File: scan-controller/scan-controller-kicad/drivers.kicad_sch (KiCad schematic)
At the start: 40 parts, among them CN2 Motor, CN3 Fan, CN4 Lamp, Q1 IRF7470, Q8 SS8050, U3 78L05, U4 DRV8871DDA, U6 TL431, U7 XL4015, U8 LM358

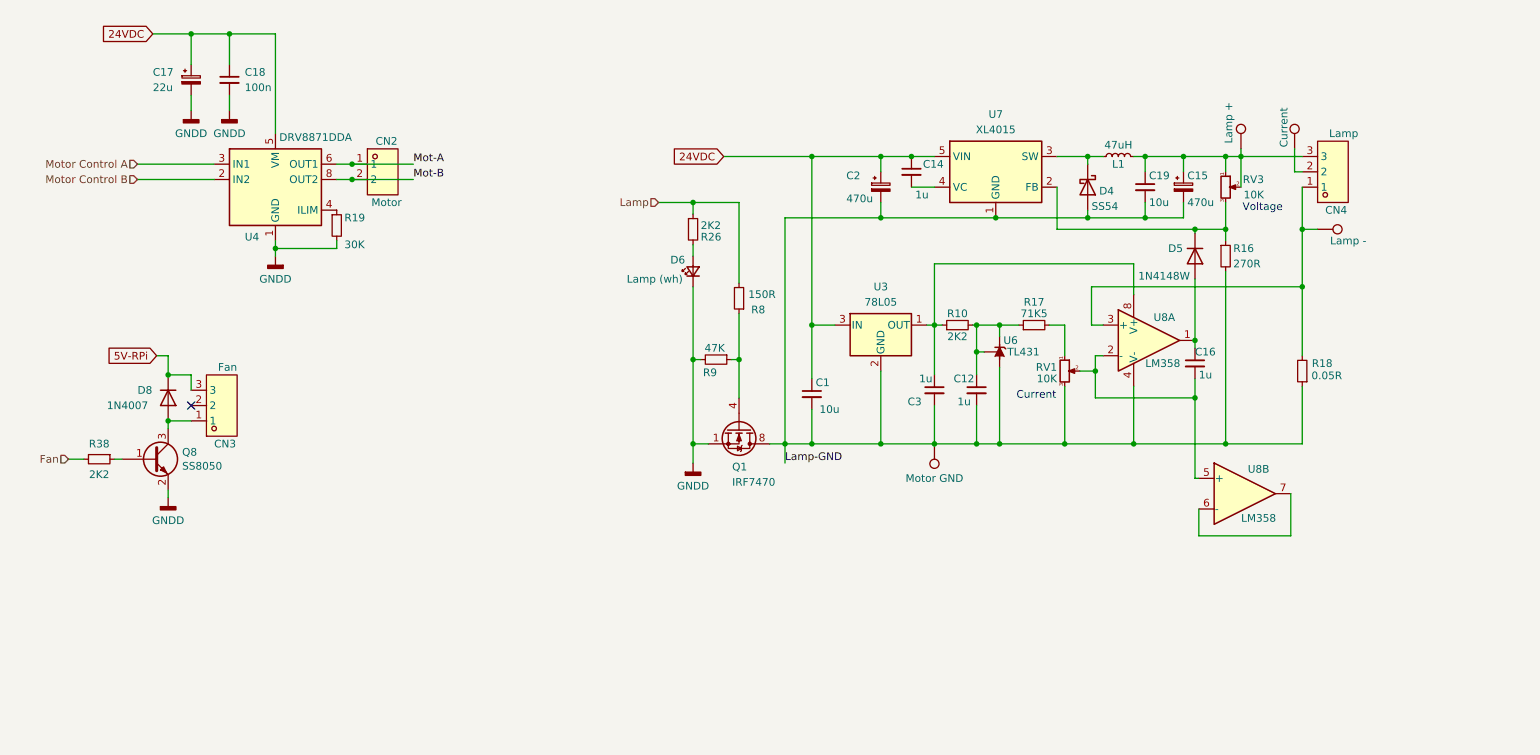
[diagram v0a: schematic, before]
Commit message: Adding a new Fan Driver (3-13V, 1A)
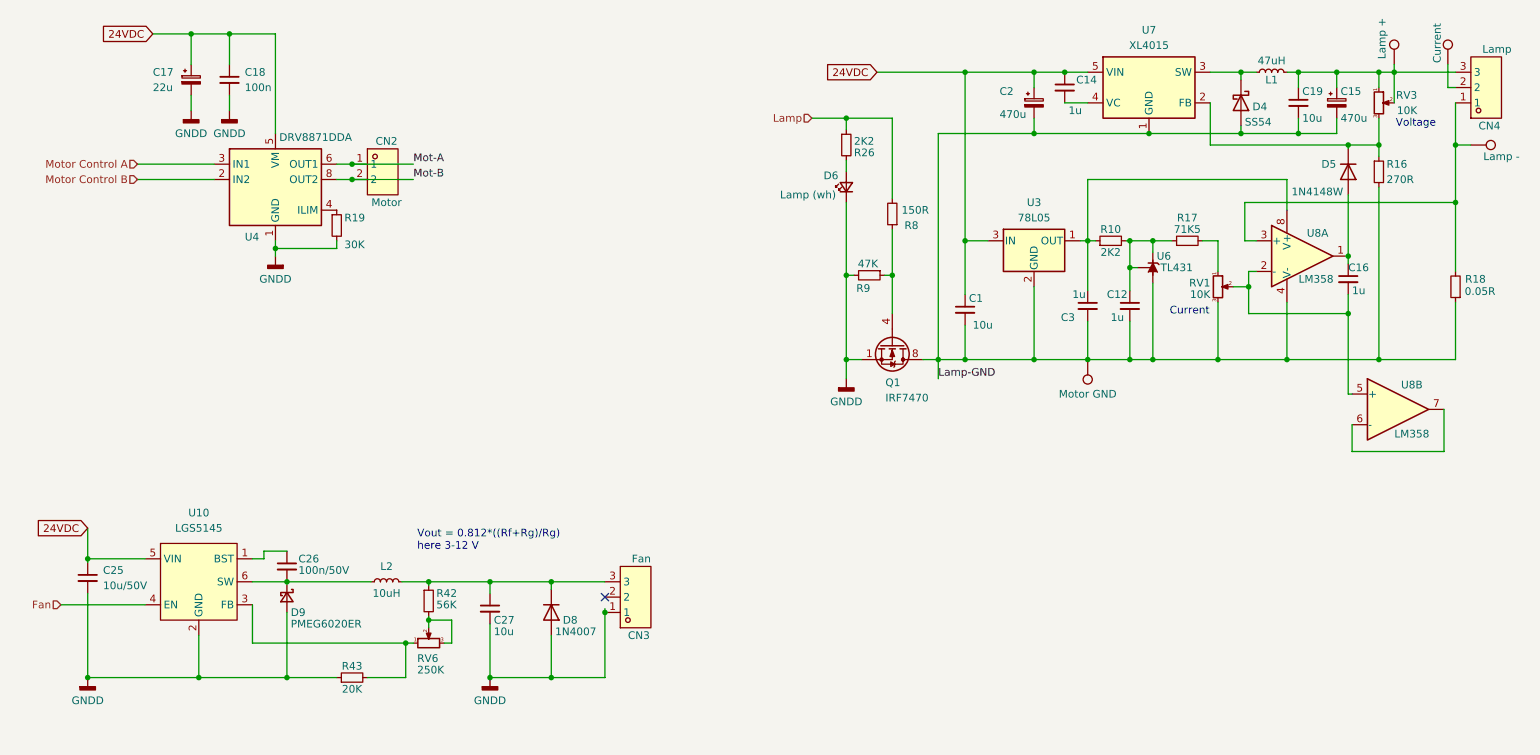
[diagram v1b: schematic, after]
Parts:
- removed Q8: SS8050, Package_TO_SOT_SMD:SOT-23, symbol Transistor_BJT:BC847
- removed R38: 2K2, Resistor_SMD:R_0805_2012Metric, symbol Device:R_Small
- added C25: 10u/50V, Capacitor_SMD:C_1210_3225Metric, symbol Device:C_Small
- added C26: 100n/50V, Capacitor_SMD:C_0805_2012Metric, symbol Device:C_Small
- added C27: 10u, Capacitor_SMD:C_0805_2012Metric, symbol Device:C_Small
- added D9: PMEG6020ER, Diode_SMD:D_SOD-123F, symbol Device:D_Schottky_Small
- added L2: 10uH, easyeda2kicad:IND-SMD_L4.4-W4.2, symbol Device:L_Small
- added R42: 56K, Resistor_SMD:R_0805_2012Metric, symbol Device:R_Small
- added R43: 20K, Resistor_SMD:R_0805_2012Metric, symbol Device:R_Small
- added RV6: 250K, easyeda2kicad:RES-ADJ-TH_3P-L10.0-W10.0-P2.50-L, symbol Device:R_Potentiometer_Small
- added U10: LGS5145, easyeda2kicad:SOT-23-6_L2.9-W1.7-P0.95-LS2.8-BL, symbol easyeda2kicad:LGS5145
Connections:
- net 24VDC: now also C25.1, U10.5 (VIN)
- net Fan: now also U10.4 (EN)
- net GNDD: now also CN3.1, D8.2 (A), C25.2, C27.2, D9.2 (A), R43.1, U10.2 (GND)
- net 5V-RPi: no longer names the net of CN3.3, D8.1 (K)
- net 5V-RPi: now also C27.1, L2.2, R42.1
- new net: C26.2, D9.1 (K), L2.1, U10.6 (SW)
- new net: R43.2, RV6.1, U10.3 (FB)
- new net: R42.2, RV6.2, RV6.3
- new net: C26.1, U10.1 (BST)
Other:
- note added: "Vout = 0.812*((Rf+Rg)/Rg) here 3-12 V"
- moved on the sheet: C1, C12, C14, C15, C16, C19, C2, C3, CN3, CN4, D4, D5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

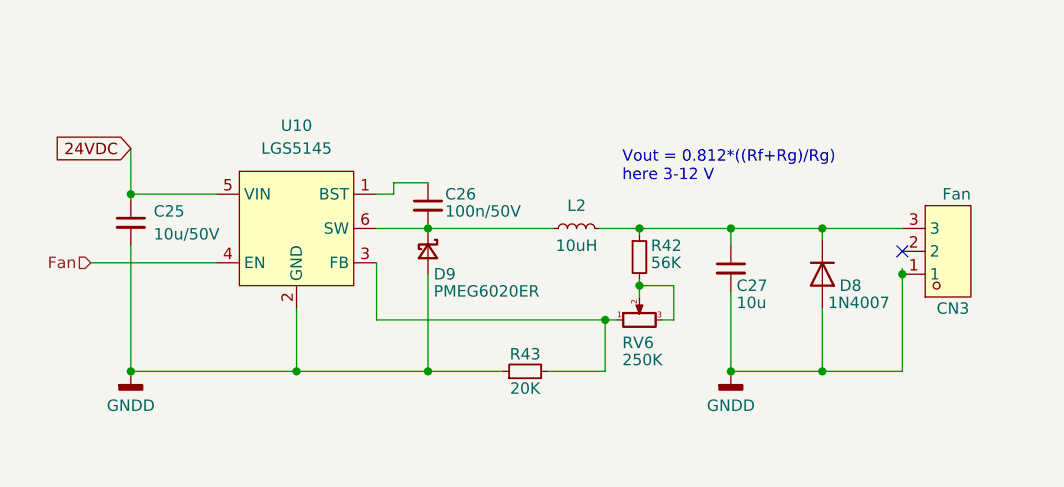
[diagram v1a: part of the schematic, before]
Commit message: Routing WIP
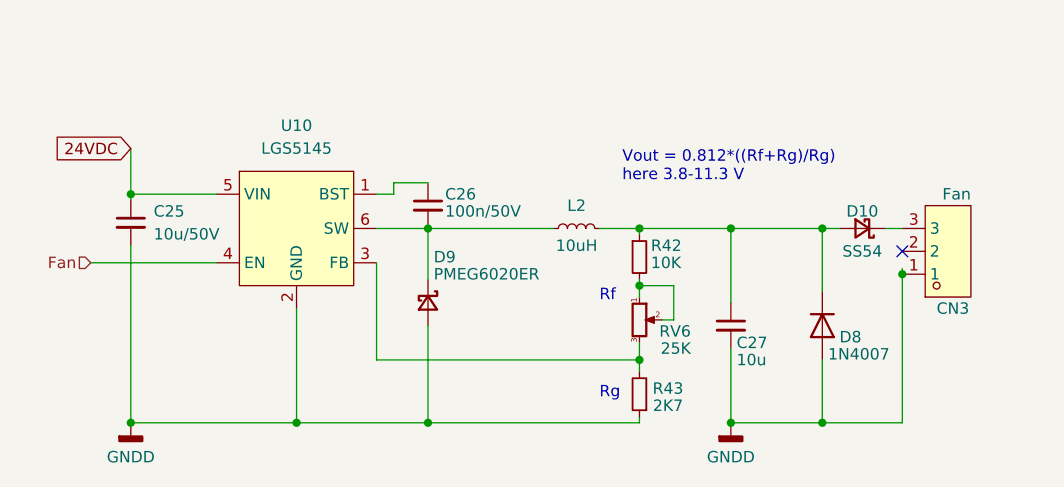
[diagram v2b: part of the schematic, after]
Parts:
- added D10: SS54, Diode_SMD:D_SMA, symbol Device:D_Schottky_Small
- R42: value 56K -> 10K; Inventory P -> B; LCSC C17756 -> C17414
- R43: value 20K -> 2K7; LCSC C4328 -> C17530
- RV6: value 250K -> 25K; LCSC C83691 -> C118932
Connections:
- net at C27.1, D8.1 (K), L2.2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: now also D10.2 (A); no longer CN3.3
- net at R43.2, U10.3 (FB): now also RV6.3; no longer RV6.1
- net at R42.2, RV6.2: now also RV6.1; no longer RV6.3
- new net: CN3.3, D10.1 (K)
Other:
- note added: "Rf"
- note added: "Rg"
- note added: "Vout = 0.812*((Rf+Rg)/Rg) here 3.8-11.3 V"
- note removed: "Vout = 0.812*((Rf+Rg)/Rg) here 3-12 V"
- moved on the sheet: C27, D8, D9, R43, RV6
